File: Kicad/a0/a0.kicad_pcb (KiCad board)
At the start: 2 copper layers, 190 x 100 mm, 122 parts, among them J1 Conn_02x03_Odd_Even, J2 VGA, J3 AudioJack4, J5 Conn_02x17_Odd_Even, J6 Barrel Jack, J7 DE9_Plug, J8 DE9_Plug, SW1 Q, SW10 P, SW11 A, SW12 S, SW13 D, SW14 F, SW15 G, SW16 H, SW17 J, SW18 K, SW19 L, SW2 W, SW20 ENTER, SW21 Z, SW22 X, SW23 C, SW24 V, SW25 SHIFT, SW26 ALT, SW27 B, SW28 N, SW29 M, SW3 E, SW30 SPACE, SW31 SW_Push, SW32 SW_SPDT, SW4 R, SW5 T, SW6 Y, SW7 U, SW8 I, SW9 O, U1 74HC590A, U10 74HC32, U11 74HC174, U12 74HC4520, U2 74HC590A, U3 CY62256-70PC, U4 SST39SF040, U5 W65C02SxP, U6 74HCT541, U7 74HC166, U8 74HC14, U9 74HC10, Y1 32Mhz

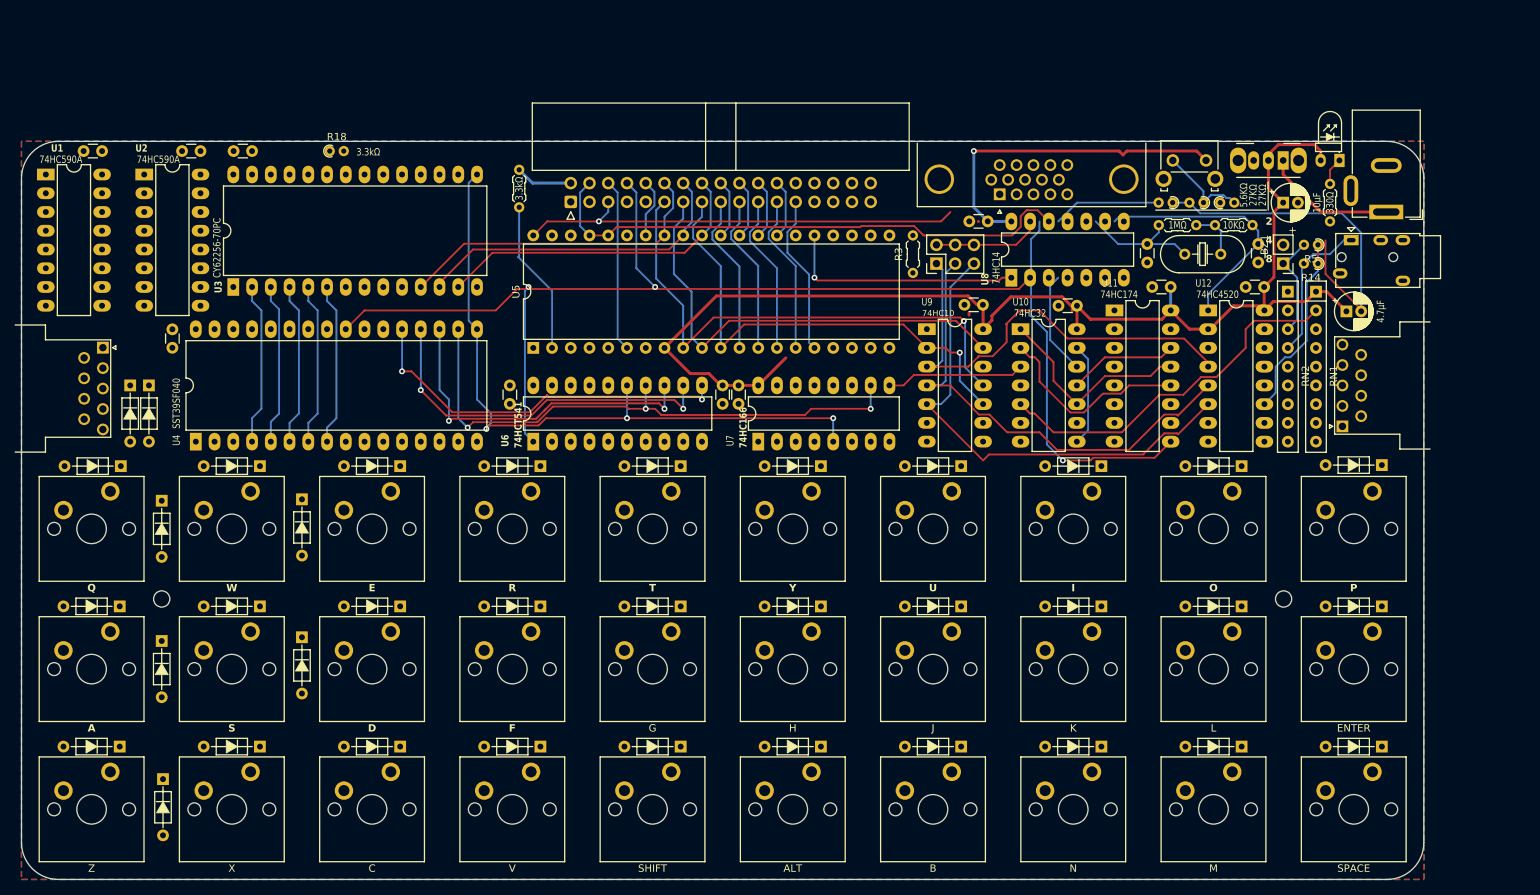
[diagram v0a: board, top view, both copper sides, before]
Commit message: Update pcb and readme
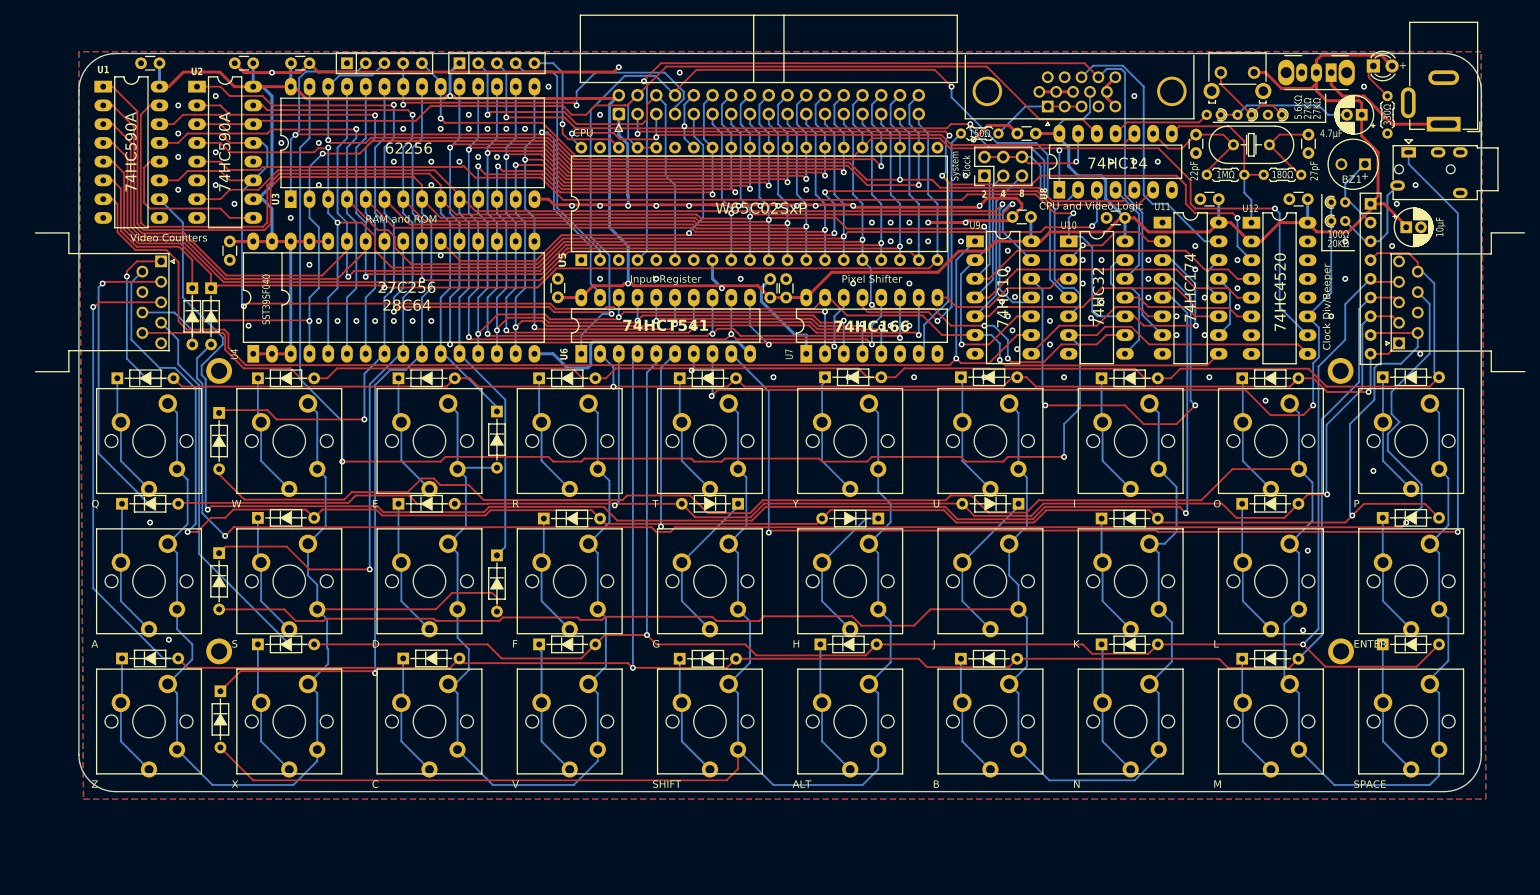
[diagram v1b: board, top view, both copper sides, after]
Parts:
- removed R18: R_Small, PCM_Resistor_THT_AKL:R_Axial_DIN0204_L3.6mm_D1.6mm_P1.90mm_Vertical
- removed R9: 3.3kΩ, PCM_Resistor_THT_AKL:R_Axial_DIN0204_L3.6mm_D1.6mm_P5.08mm_Horizontal
- added H3: MountingHole_Pad, MountingHole:MountingHole_2.2mm_M2_ISO7380_Pad, F.Cu at (74.3, 111.6)
- added H4: MountingHole_Pad, MountingHole:MountingHole_2.2mm_M2_ISO7380_Pad, F.Cu at (226.3, 111.6)
- added RN3: R_Network04, Resistor_THT:R_Array_SIP5, F.Cu at (91.6, 31.9)
- BZ1: footprint Connector_PinHeader_2.54mm:PinHeader_1x02_P2.54mm_Vertical -> Buzzer_Beeper:MagneticBuzzer_Kingstate_KCG0601
- C1: value 33pF -> 22pF
- C2: value 33pF -> 27pF
- D1: footprint PCM_LED_THT_AKL_Double:LED_D3.0mm_Horizontal_O1.27mm_Z2.0mm_IRGrey -> LED_THT:LED_D3.0mm
- H1, H2: value MountingHole -> MountingHole_Pad; footprint MountingHole:MountingHole_2.2mm_M2 -> MountingHole:MountingHole_2.2mm_M2_ISO7380_Pad
- J7, J8: footprint Connector_Dsub:DSUB-9_Male_Horizontal_P2.77x2.54mm_EdgePinOffset9.40mm -> Smal:DSUB9-Atari
- R2: value 10KΩ -> 180Ω
- RN2: value R_Network08 -> R_Network04; footprint Resistor_THT:R_Array_SIP9 -> Resistor_THT:R_Array_SIP5
- SW1, SW10, SW11, SW12, SW13, SW14, SW15, SW16, SW17, SW18, SW19, SW2, SW20, SW21, SW22, SW23, SW24, SW25, SW26, SW27, SW28, SW29, SW3, SW30, SW4, SW5, SW6, SW7, SW8, SW9: footprint PCM_Switch_Keyboard_Cherry_MX:SW_Cherry_MX_PCB_1.00u -> Smal:SW_Redragon_MX_LowProfile_PCB_1.00u_Other
- U3: value CY62256-70PC -> 62256
- moved H1 162.7 mm to (226.2, 73.6)
- moved H2 147.5 mm to (74.3, 73.6)
- moved RN2 116.4 mm to (106.8, 31.9), turned to 0 degrees
- moved D3 29.0 mm to (111.9, 79.1)
- moved D2 28.7 mm to (111.9, 98.6)
- moved C3 26.7 mm to (229.1, 38.9), turned to 180 degrees
- moved R3 20.0 mm to (174.8, 41.4), turned to 0 degrees
- moved C8 18.1 mm to (120.2, 61.1), turned to -90 degrees
- moved BZ1 17.4 mm to (229.5, 45.6)
- moved C10 17.4 mm to (148.9, 61.2), turned to -90 degrees
- moved C16 17.0 mm to (235.1, 54.1)
- moved C2 16.3 mm to (221.9, 41.6)
- moved Y1 16.2 mm to (211.7, 43.0)
- moved C1 16.2 mm to (206.6, 41.6)
- moved D19 15.9 mm to (144.6, 91.6)
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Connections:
- C2 pad 1: Net-(U12A-CK) -> Net-(C2-Pad1)
- J2 pad 13: /~{HSYNC} -> /~{HSYNC}**
- J2 pad 9: GND -> VCC
- J3 pad R1: GND -> unconnected-(J3-PadR1)
- J3 pad R2: unconnected-(J3-PadR2) -> GND
- J3 pad S: /AUDIN -> /DataOut
- J3 pad T: /DataOut -> /AUDIN
- J5 pad 4: ø2 -> /ø2
- R1 pad 2: Net-(R1-Pad2) -> Net-(U12A-CK)
- R13 pad 1: GND -> Net-(R12-Pad1)
- R13 pad 2: Net-(R12-Pad1) -> GND
- R2 pad 1: Net-(R1-Pad2) -> Net-(C2-Pad1)
- RN1 pad 2: /r/~{w} -> /Speaker
- RN1 pad 3: /NMI -> /DataOut
- RN1 pad 4: /HROW 0 -> /HROW 5
- RN1 pad 5: /HROW 1 -> /HROW 3
- RN1 pad 7: /HROW 3 -> /HROW 1
- RN1 pad 9: /HROW 5 -> /HROW 0
- RN2 pad 1: GND -> VCC
- RN2 pad 2: unconnected-(RN2-R1-Pad2) -> /~{NMI}
- RN2 pad 3: /Speaker -> /r/~{w}
- RN2 pad 4: /DataOut -> /RDY
- RN2 pad 5: /A13 -> /~{SO}
- U1 pad 11: /M2 -> /~{sload}
- U1 pad 13: /M2 -> /~{sload}
- U1 pad 14: ø2 -> /ø2
- U10 pad 11: Net-(U11-D5) -> Net-(U11-D3)
- U11 pad 10: /~{VSYNC} -> /~{HSYNC}
- U11 pad 12: /H32' -> /~{HSYNC}*
- U11 pad 13: /H32 -> /~{HSYNC}
- U11 pad 14: Net-(U11-D5) -> /~{HSYNC}*
- U11 pad 15: /~{HSYNC} -> /~{HSYNC}**
- U11 pad 2: unconnected-(U11-Q0-Pad2) -> /H32'
- U11 pad 3: unconnected-(U11-D0-Pad3) -> /H32
- U11 pad 4: /V512 -> Net-(U11-D1)
- U11 pad 5: /V512' -> /~{MRC}
- U11 pad 7: /~{MRC} -> /~{VSYNC}
- U11 pad 9: ø2 -> /~{sload}
- U2 pad 10: /~{MRC} -> VCC
- U2 pad 11: /M2 -> /~{sload}
- U2 pad 13: /M2 -> /~{sload}
- U2 pad 14: ø2 -> /ø2
- U2 pad 6: /A1 -> unconnected-(U2-Q6-Pad6)
- U4 pad 28: /A13 -> VCC
- U4 pad 29: /A14 -> VCC
- U5 pad 2: Net-(U5-RDY) -> /RDY
- U5 pad 36: ø2 -> /ø2
- U5 pad 37: ø2 -> /ø2
- U5 pad 38: VCC -> /~{SO}
- U7 pad 6: /V512' -> GND
- U8 pad 12: ø2 -> /ø2
- U9 pad 12: Net-(U11-D2) -> Net-(U11-D1)
- U9 pad 8: Net-(U11-D3) -> Net-(U11-D2)
- Y1 pad 2: Net-(R1-Pad2) -> Net-(C2-Pad1)
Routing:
- net /HROW 2: track 0.00 -> 318.6 mm, vias 0 -> 2
- net /HROW 3: track 0.00 -> 310.2 mm, vias 0 -> 2
- net /COL 4: track 0.00 -> 283.6 mm
- net /HROW 4: track 0.00 -> 280.5 mm, vias 0 -> 3
- net /HROW 1: track 0.00 -> 259.0 mm, vias 0 -> 3
- net /COL 3: track 0.00 -> 238.8 mm
- net Net-(D37-A): track 0.00 -> 227.5 mm, vias 0 -> 2
- net /A2: track 65.4 -> 288.2 mm, vias 1 -> 4
- net /~{MRC}: track 0.00 -> 216.6 mm, vias 0 -> 2
- net GND: track 0.00 -> 213.7 mm, vias 0 -> 124
- net /HROW 5: track 0.00 -> 211.7 mm, vias 0 -> 1
- net /HROW 0: track 0.00 -> 206.6 mm, vias 0 -> 3
- net /~{WR}: track 0.00 -> 205.9 mm, vias 0 -> 2
- net /COL 2: track 0.00 -> 203.4 mm
- net /~{sload}: track 0.00 -> 191.8 mm, vias 0 -> 2
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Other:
- board text added: "27C256 28C64"
- board text added: "CPU"
- board text added: "CPU and Video Logic"
- board text added: "Clock Div/Beeper"
- board text added: "Input Register"
- board text added: "MicroMicro v0 - Dec 2024"
- board text added: "Pixel Shifter"
- board text added: "RAM and ROM"
- board text added: "System Clock"
- board text added: "Video Counters"
- board text added: "github.com/smaldragon/MicroMicro"
- board text removed: "3.3kΩ"
